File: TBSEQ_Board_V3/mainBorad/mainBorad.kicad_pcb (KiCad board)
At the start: 2 copper layers, 201 x 150 mm, 263 parts, among them IC1 NJM2125F-TE1_DIP8, IC12 4066, IC2 NJM2125F-TE1, IC3 74AHC1G04W5-7, IC4 NJM2125F-TE1, IC5 NJM2125F-TE1_DIP8, J1 Conn_01x08, J10 Conn_01x05, J11 Conn_01x05, J12 Conn_01x02, J13 Conn_01x01_Pin, J14 Conn_01x05, J3 Conn_01x02_Pin, J4 Conn_01x02, J5 Conn_01x02, J6 MJ-462, J7 Conn_01x03_Pin, J8 Conn_01x02_Pin, J9 Conn_01x01_Pin, Q1 NPN, Q10 PNP, Q11 NPN, Q12 HN1C01FU-GR,LF, Q13 NPN, Q14 NPN, Q15 NPN, Q16 NPN, Q17 NPN, Q18 NPN, Q19 NPN, Q2 PNP, Q20 NPN, Q21 HN1C01FU-GR,LF, Q22 HN1C01FU-GR,LF, Q23 NPN, Q24 NPN, Q25 NPN, Q26 HN1C01FU-GR,LF, Q27 PNP, Q28 NJFET, Q29 NPN, Q30 NPN, Q35 NPN, Q36 PNP, Q37 NPN, Q38 PNP, Q39 NJFET, Q4 2SC3325-Y, Q40 NPN, Q41 NPN, Q8 PNP, Q9 PNP, SW1 2MS1T1B4VS2QES, U1 LM13700

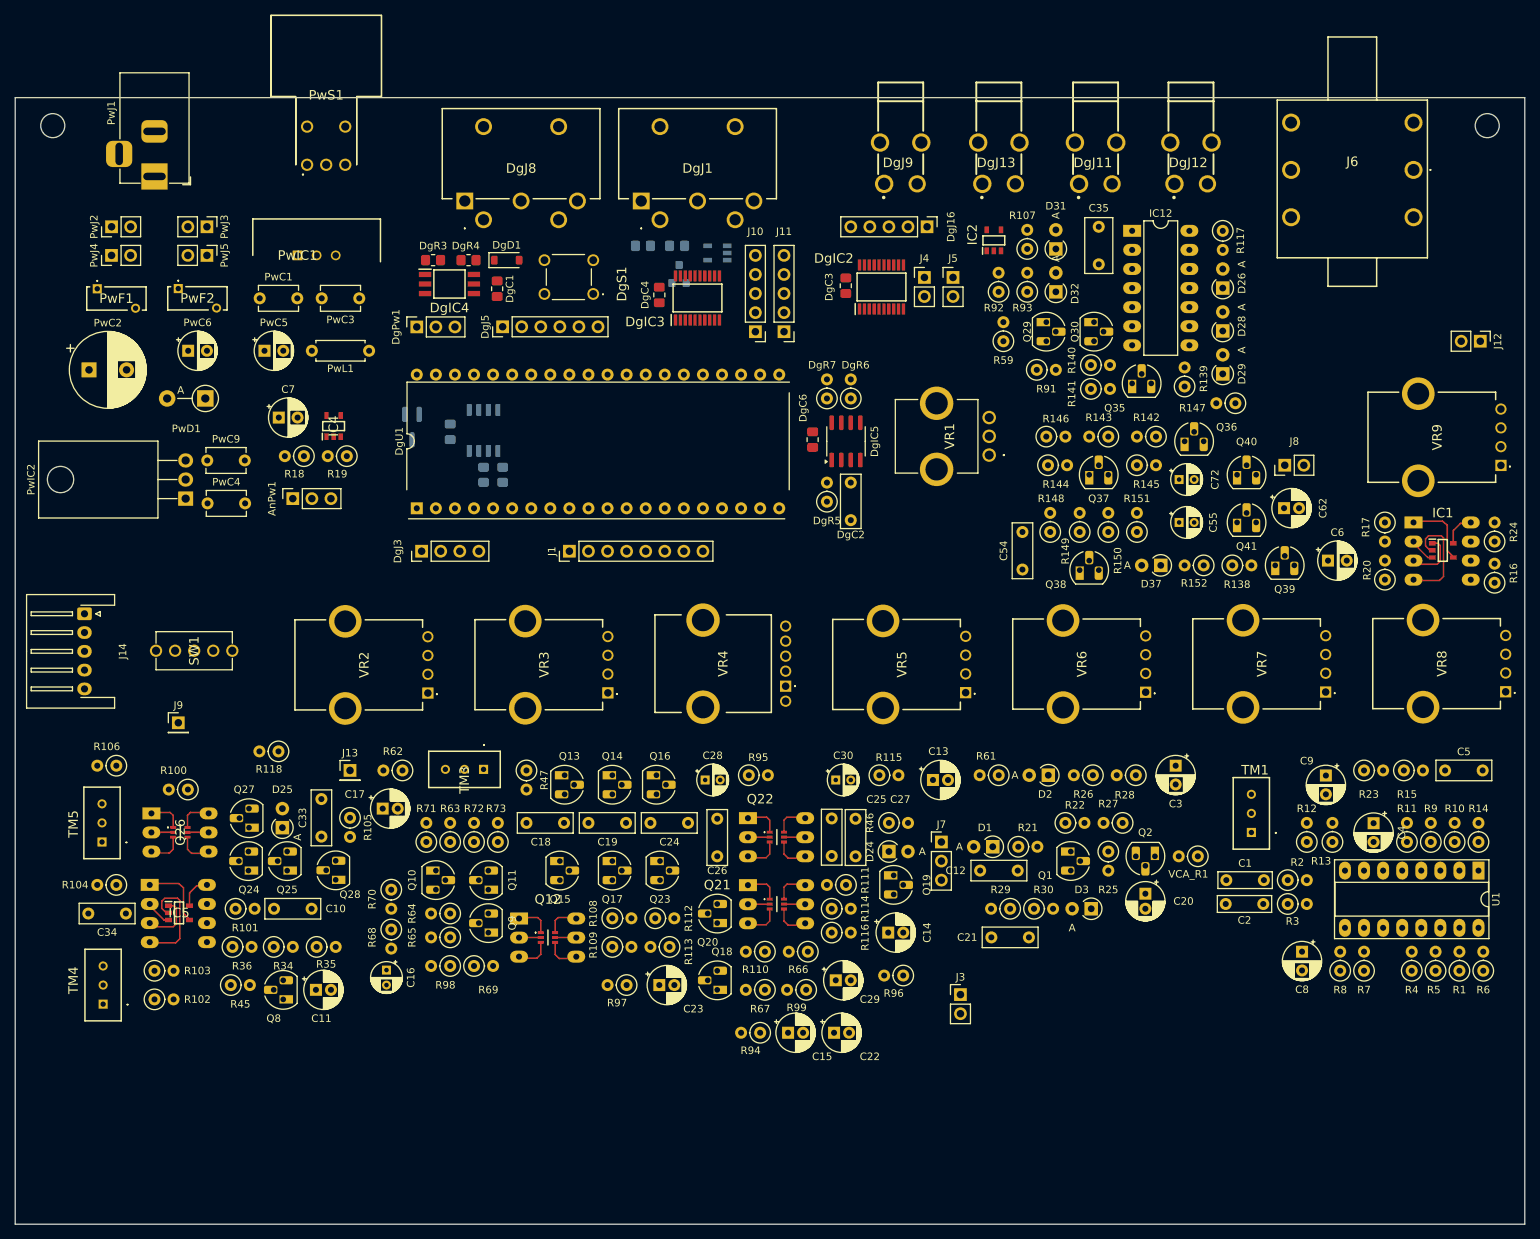
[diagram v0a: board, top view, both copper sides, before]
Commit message: V3Board
GNDパターン塗り済
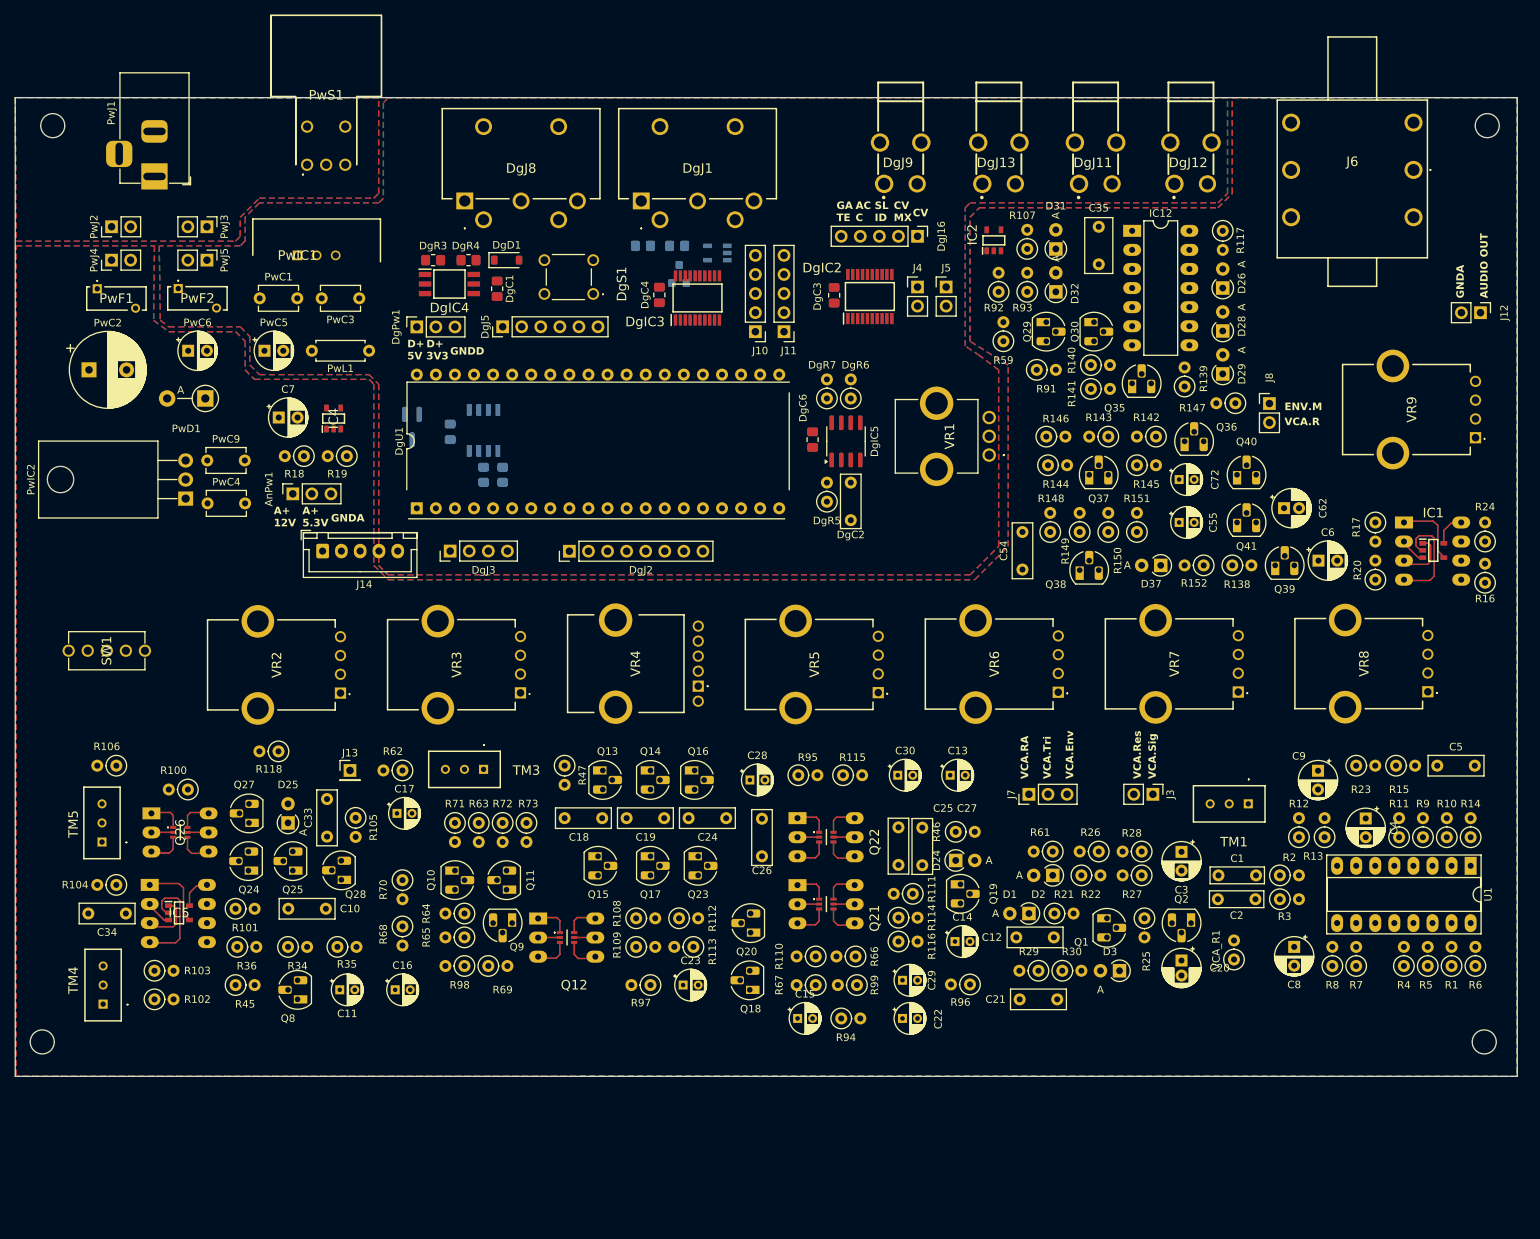
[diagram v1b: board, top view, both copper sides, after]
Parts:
- removed J9: Conn_01x01_Pin, Connector_PinHeader_2.54mm:PinHeader_1x01_P2.54mm_Vertical
- C11, C13, C14, C15, C17, C22, C23, C29: footprint Capacitor_THT:CP_Radial_D5.0mm_P2.00mm -> Capacitor_THT:CP_Radial_D4.0mm_P2.00mm
- J14: footprint Connector_JST:JST_XH_S5B-XH-A-1_1x05_P2.50mm_Horizontal -> Connector_JST:JST_XH_B5B-XH-A_1x05_P2.50mm_Vertical
- moved J3 37.0 mm to (175.5, 113.0), turned to -90 degrees
- moved J14 32.8 mm to (64.9, 80.6), turned to 0 degrees
- moved VCA_R1 14.6 mm to (186.3, 135.0), turned to 90 degrees
- moved D2 13.3 mm to (162.2, 123.8)
- moved J7 13.3 mm to (159.0, 113.0), turned to 90 degrees
- moved R61 12.4 mm to (162.2, 120.7)
- moved VR5 11.6 mm to (138.9, 99.5)
- moved VR4 11.6 mm to (114.9, 98.6)
- moved SW1 11.6 mm to (33.7, 93.9)
- moved VR2 11.6 mm to (67.3, 99.5)
- moved VR3 11.6 mm to (91.3, 99.5)
- moved VR6 11.6 mm to (162.9, 99.4)
- moved VR7 11.6 mm to (186.9, 99.4)
- moved C3 11.5 mm to (179.3, 120.7)
- moved R94 11.0 mm to (134.0, 142.9), turned to 0 degrees
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- renumbered J1 to DgJ2
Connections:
- DgJ11 pad 2: A+CV_MIX -> A+VCO_CV
- DgJ11 pad 3: A+CV_MIX -> A+VCO_CV
- DgJ16 pad 2: A+CV_MIX -> A+VCO_CV
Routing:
- added copper zone on B.Cu, net ADAPTER GND
- added copper zone on F.Cu, net ADAPTER GND
- added copper zone on B.Cu, net GNDA
- added copper zone on F.Cu, net GNDA
- added copper zone on B.Cu, net GNDD
- added copper zone on F.Cu, net GNDD
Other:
- board size 201 x 150 mm -> 200 x 130.3 mm
- board text added: "A+ 12V"
- board text added: "A+ 5.3V"
- board text added: "AC C"
- board text added: "AUDIO OUT"
- board text added: "CV"
- board text added: "CV MX"
- board text added: "D+ 3V3"
- board text added: "D+ 5V"
- board text added: "ENV.M"
- board text added: "GA TE"
- board text added: "GNDA"
- board text added: "GNDD"
- board text added: "SL ID"
- board text added: "VCA.Env"
- board text added: "VCA.R"
- board text added: "VCA.RA"
- board text added: "VCA.Res"
- board text added: "VCA.Sig"
- board text added: "VCA.Tri"
